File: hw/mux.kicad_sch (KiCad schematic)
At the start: 5 parts, among them U11 NCP708, U14 BL1530TQFN

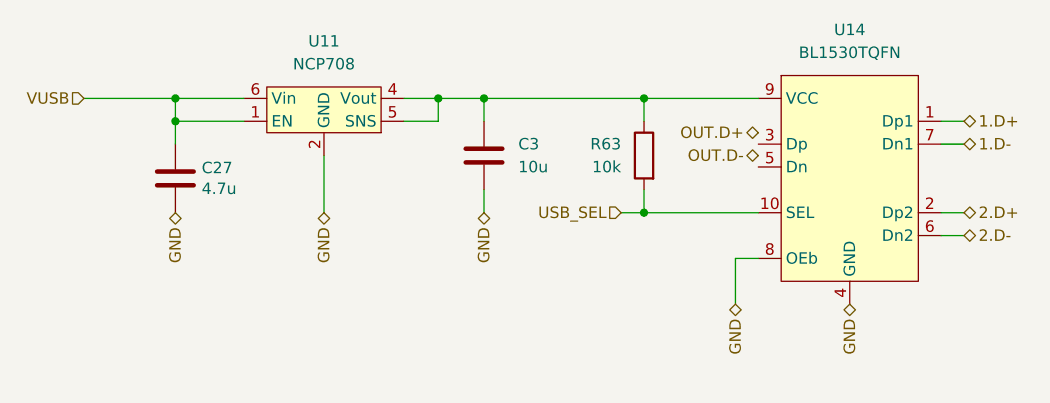
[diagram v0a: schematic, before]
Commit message: Mišmaš
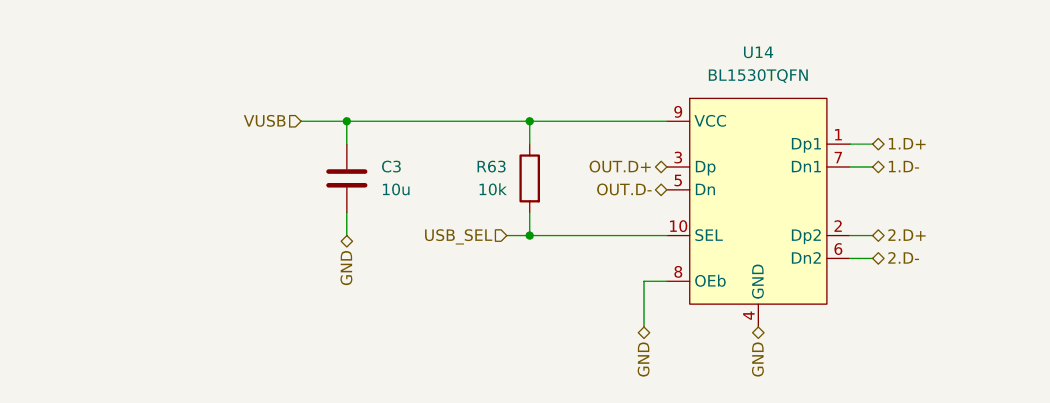
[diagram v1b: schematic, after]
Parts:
- removed C27: 4.7u, Capacitor_SMD:C_0603_1608Metric, symbol Device:C
- removed U11: NCP708, RKL-StandardPackages:UDFN6-3x3mm, symbol RKL-LDO:NCP708
- C3: Price (100ks) (none) -> 0.0159; Price (1ks) (none) -> 0.0159
- R63: Price (100ks) (none) -> 0.0005; Price (1ks) (none) -> 0.0005
- U14: Basic/Extended (none) -> E; Price (100ks) (none) -> 0.1148; Price (1ks) (none) -> 0.1445
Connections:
- net OUT.D+: now also U14.3 (Dp)
- net OUT.D-: now also U14.5 (Dn)
- net VUSB: now also C3.1, R63.1, U14.9 (VCC)
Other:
- moved on the sheet: C3, R63, U14
